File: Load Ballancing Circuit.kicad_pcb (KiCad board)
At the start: 2 copper layers, 33 x 39 mm, 38 parts, among them J2 171857-0005, J3 171857-0004, J4 171857-0006, U1 LTC4359HMS8#PBF, U2 LTC4359HMS8#PBF, U3 INA139, U4 MAX11615, U5 INA139

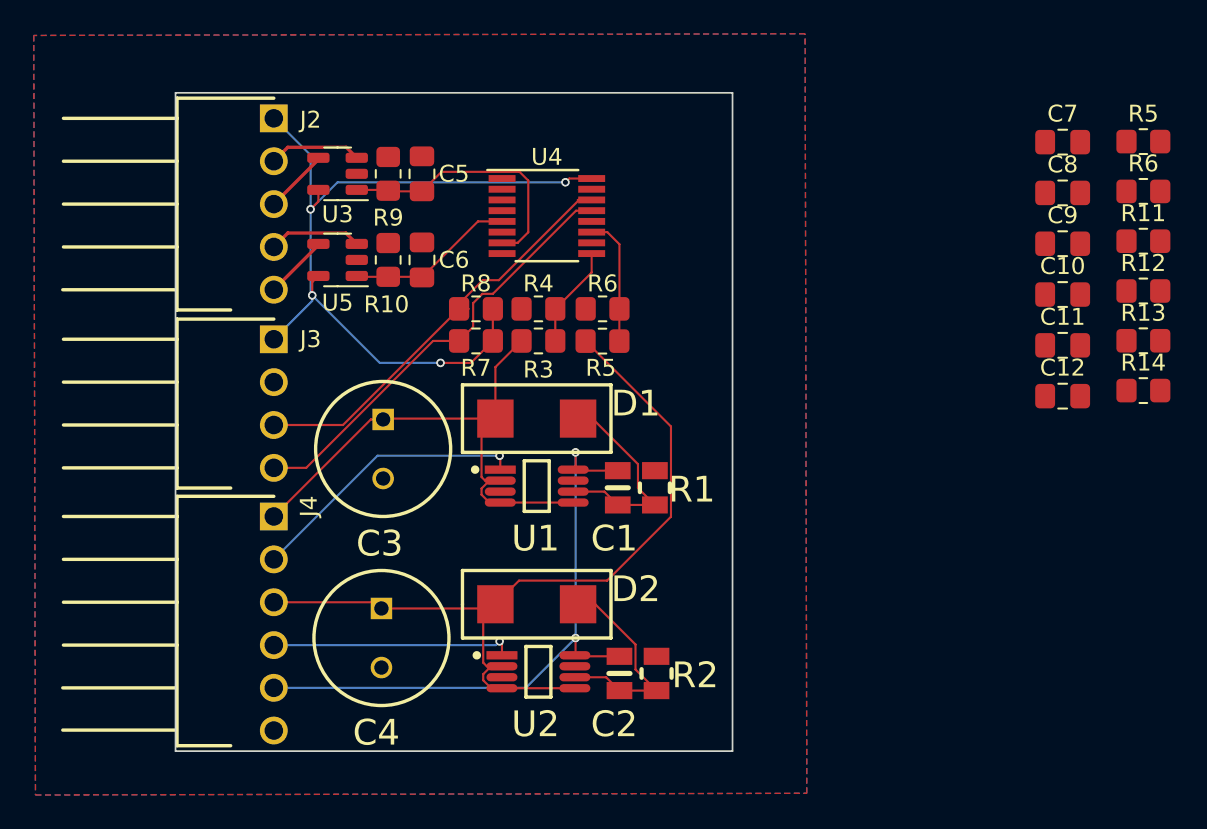
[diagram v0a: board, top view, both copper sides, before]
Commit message: changed circuit
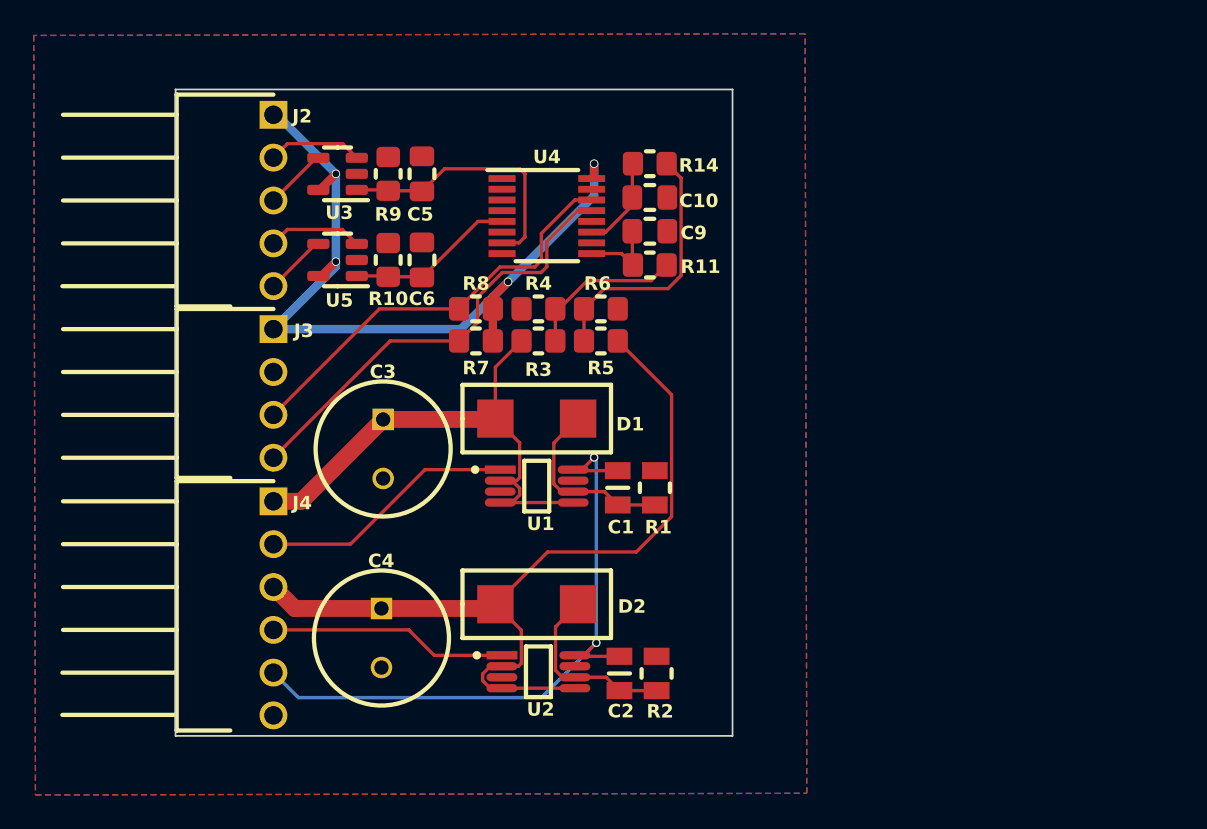
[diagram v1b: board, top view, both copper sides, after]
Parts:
- removed C11, C12, C7, C8: 10uF, Capacitor_SMD:C_0805_2012Metric_Pad1.18x1.45mm_HandSolder
- removed R12, R13: 1k, Resistor_SMD:R_0805_2012Metric_Pad1.20x1.40mm_HandSolder
- removed the R5 at (175.1, 86.6)
- removed the R5 at (207.2, 74.8)
- removed the R6 at (207.2, 77.8)
- removed the R6 at (175.2, 84.7)
- added R5: 10M, Resistor_SMD:R_0805_2012Metric_Pad1.20x1.40mm_HandSolder, F.Cu at (175.1, 86.6)
- added R6: 1.38M, Resistor_SMD:R_0805_2012Metric_Pad1.20x1.40mm_HandSolder, F.Cu at (175.1, 84.7)
- moved R14 32.2 mm to (178.0, 76.1)
- moved R11 29.3 mm to (178.0, 82.1)
- moved C10 25.1 mm to (178.0, 78.1), turned to 180 degrees
- moved C9 24.5 mm to (178.0, 80.1), turned to 180 degrees
- moved J4 0.90 mm to (157.0, 94.7)
- moved J3 0.60 mm to (157.0, 84.5)
- moved J2 0.21 mm to (157.0, 71.8)
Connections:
- U4 pad 10: Net-(U4-AIN5) -> GND
- U4 pad 12: Net-(U4-AIN7) -> GND
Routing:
- net Net-(R14-Pad2): track 0.00 -> 15.4 mm
- net Net-(R11-Pad2): track 0.00 -> 9.58 mm
- net /V_BAT_OUT: track 37.6 -> 40.6 mm
- net Net-(U4-AIN6): track 7.68 -> 5.55 mm
- net 3V3: track 49.8 -> 47.7 mm
- net Net-(D2-2): track 12.8 -> 11.0 mm
- net Net-(D1-2): track 12.7 -> 11.0 mm
- net /GATE_1: track 16.8 -> 15.3 mm, vias 1 -> 0
- net Net-(U4-AIN4): track 6.07 -> 4.74 mm
- net /I2C_SDA: track 25.9 -> 25.1 mm
- net /I2C_SCL: track 26.0 -> 26.7 mm
- net /GATE_2: track 14.4 -> 14.2 mm, vias 1 -> 0
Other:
- board size 33 x 39 mm -> 33 x 38.3 mm
